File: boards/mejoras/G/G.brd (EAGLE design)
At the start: 100 x 45 mm, 34 parts, among them J1 XT60-M, J2 XT60-M, J3 XT60-M, J4 XT60-M, J5 XT60-M, J6 XT60-M, Q1 IRFR7440PBF, Q2 IRFR7440PBF

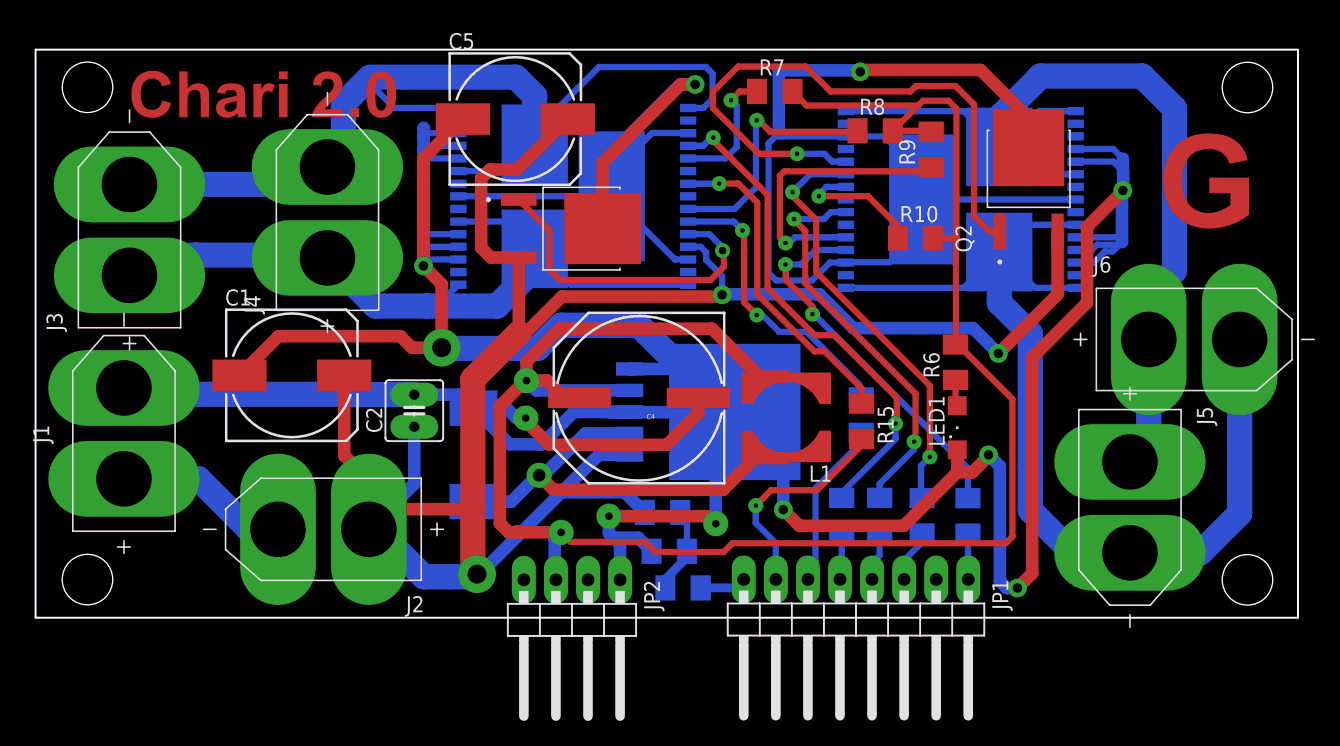
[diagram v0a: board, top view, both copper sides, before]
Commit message: changes to g circuit
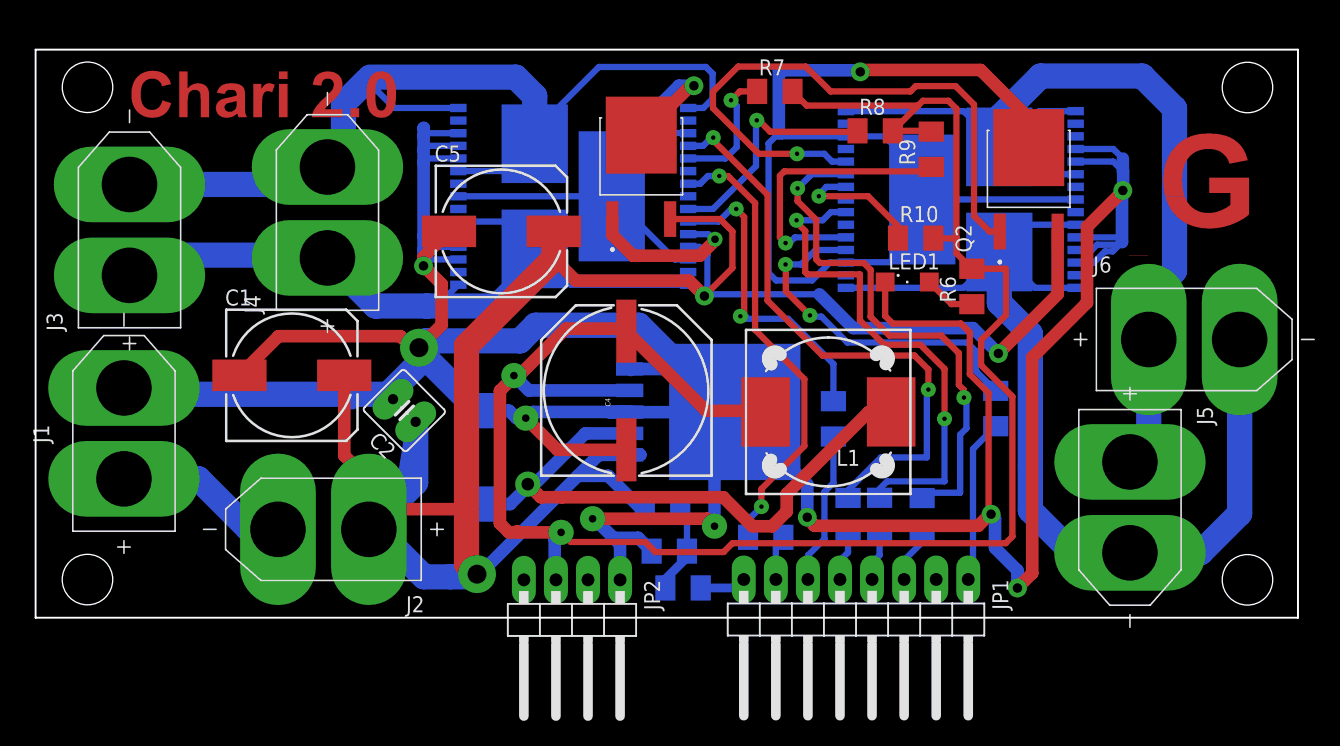
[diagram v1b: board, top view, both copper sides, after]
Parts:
- L1: value MSS7341 -> DR125; device inductor-coilcraft:MSS7341 -> inductors:DR125
- moved LED1 12.2 mm to (69.0, 26.6), turned to 0 degrees
- moved R15 11.9 mm to (57.8, 6.37), flipped to the bottom, turned to 180 degrees
- moved C5 8.97 mm to (36.9, 30.6)
- moved R2 8.78 mm to (76.1, 16.6)
- moved Q1 7.41 mm to (48.0, 35.7), turned to 90 degrees
- moved R6 6.14 mm to (74.2, 26.2)
- moved L1 3.36 mm to (62.8, 16.3)
- moved R5 2.22 mm to (63.2, 15.8)
- moved C4 1.17 mm to (46.8, 18.0), turned to 90 degrees
- moved C2 0.79 mm to (29.2, 16.4), turned to 135 degrees
- moved R4 0.50 mm to (64.4, 8.09)
- moved D2 0.45 mm to (35.1, 12.7)
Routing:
- net PWM2: track 17.4 -> 3.86 mm, vias 1 -> 0
- net N$13: track 35.7 -> 49.2 mm
- net N$1: track 25.9 -> 13.0 mm
- net N$16: track 59.2 -> 47.9 mm
- net N$14: track 26.3 -> 36.4 mm, vias 1 -> 2
- net IN1A: track 3.65 -> 13.0 mm
- net N$15: track 31.6 -> 39.9 mm
- net N$12: track 33.9 -> 42.0 mm
- net N$9: track 39.6 -> 46.9 mm
- net VPOWER: track 165.7 -> 168.8 mm
- net N$4: track 2.10 -> 4.09 mm
- net N$11: track 29.8 -> 28.2 mm
- net N$10: track 23.9 -> 25.4 mm
- net 5V: track 154.8 -> 153.3 mm
- net N$5: track 19.8 -> 18.8 mm
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
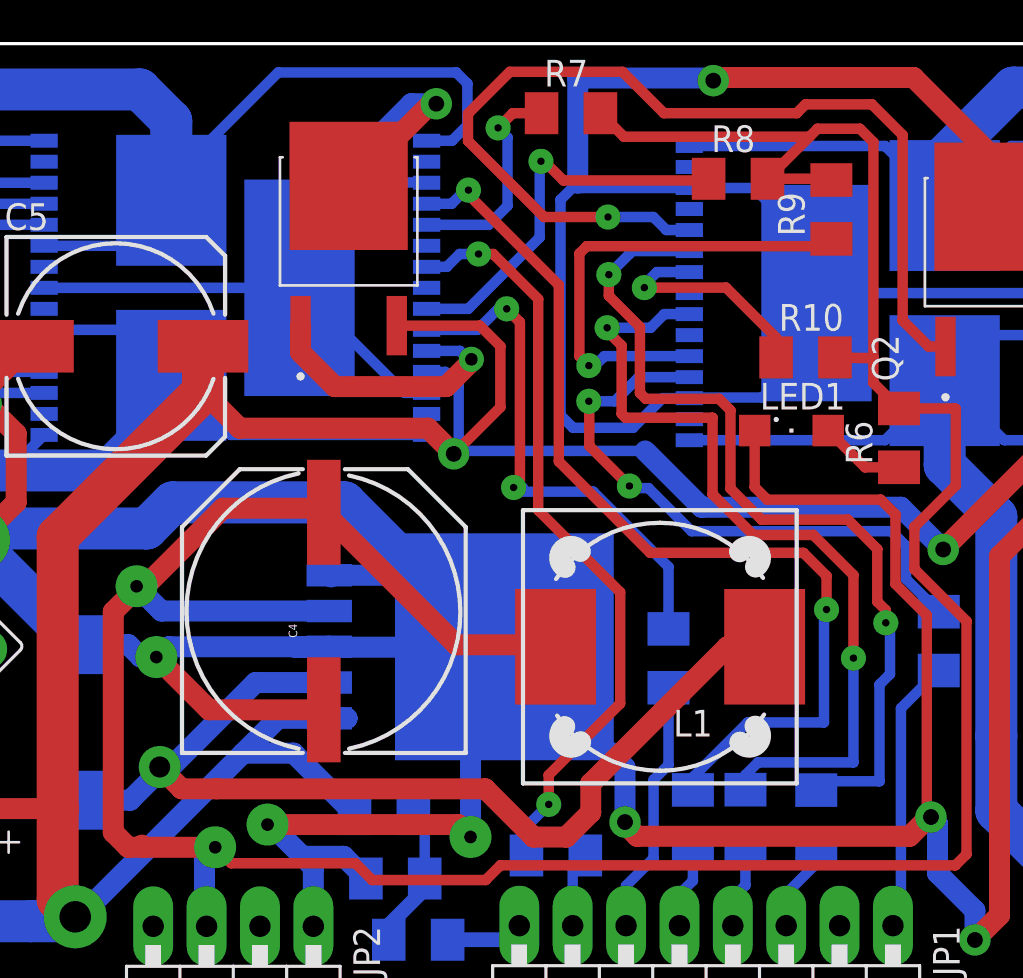
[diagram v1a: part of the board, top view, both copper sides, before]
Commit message: corrected bug
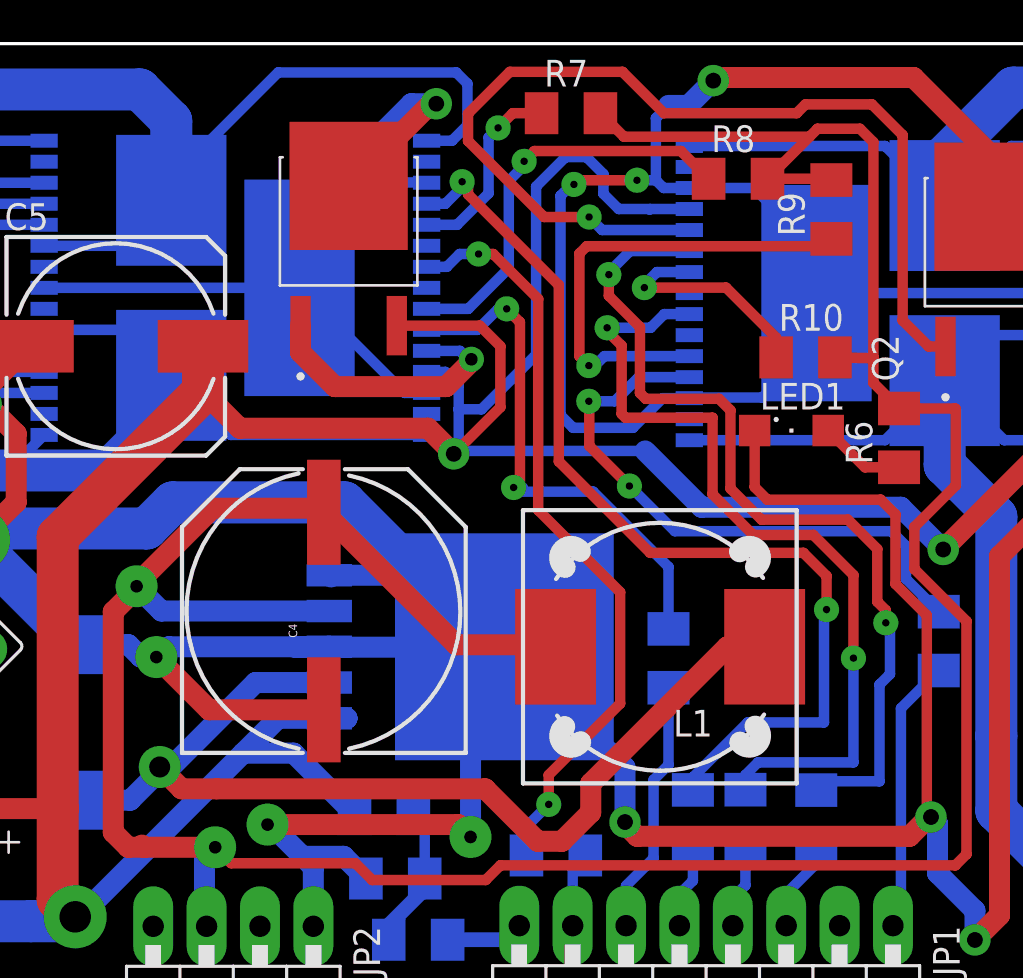
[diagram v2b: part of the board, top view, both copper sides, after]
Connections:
- removed net POWER: U$2.12
- net VPOWER: now also U$2.12
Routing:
- net VPOWER: track 168.8 -> 191.0 mm
- net N$18: track 83.8 -> 79.0 mm, vias 1 -> 3
- net N$2: track 10.5 -> 9.23 mm
- net N$5: track 18.8 -> 19.6 mm
- net N$9: track 46.9 -> 47.4 mm
